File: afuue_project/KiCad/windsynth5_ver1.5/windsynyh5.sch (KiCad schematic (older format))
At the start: 35 parts, among them P1 SENSOR, P2 SPEAKER, P3 HEADPHONE, P4 EXT-POWER, P5 EXT, P6 AE-PAM8012, P7 I2C, P8 MIDI-TRS, U1 ESP32-DEVKIT-C, U2 TDA1543, U3 TDA1543

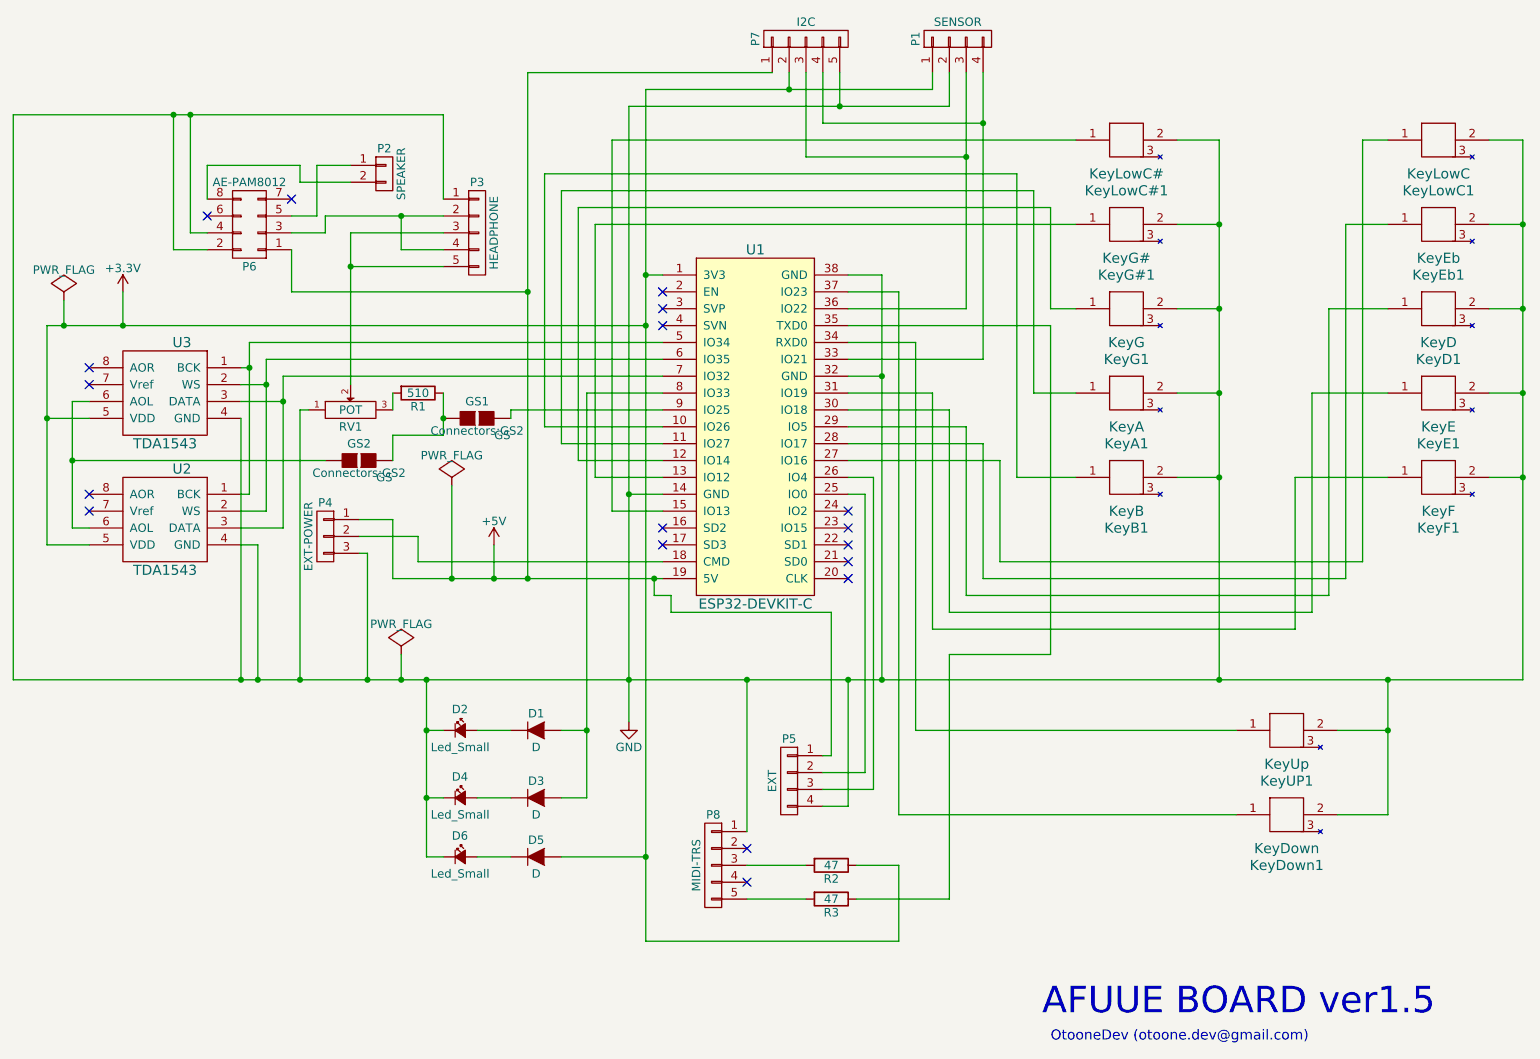
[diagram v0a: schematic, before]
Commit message: 現状のものを一旦コミット（KORG NTS-1対応含む）
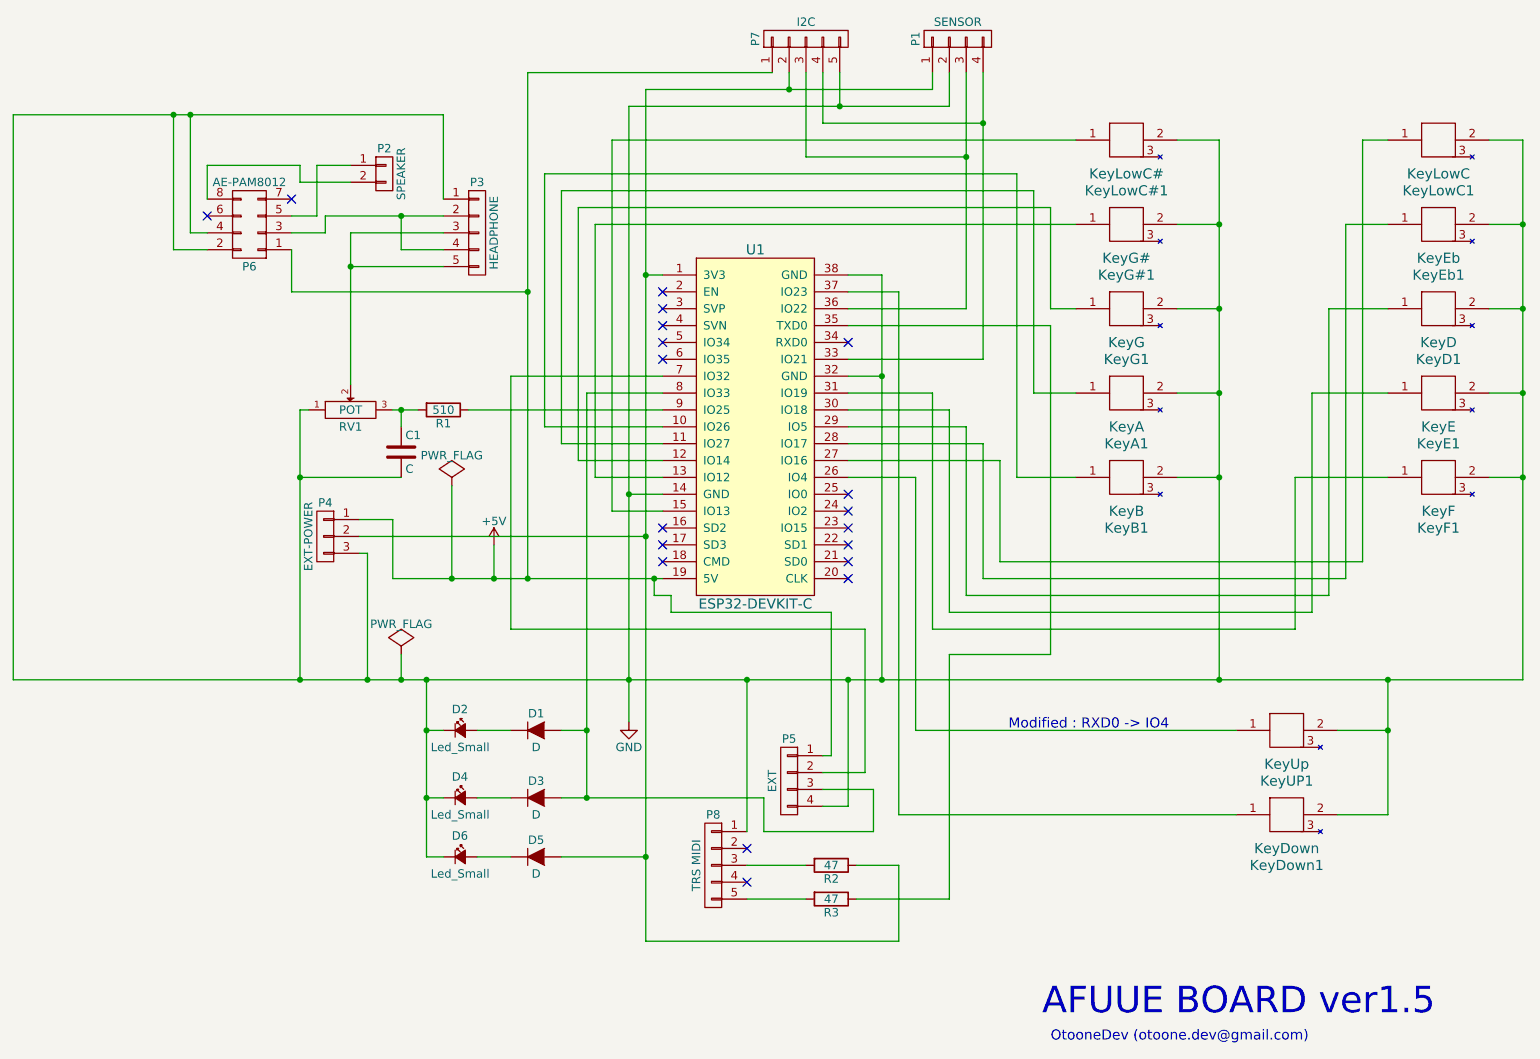
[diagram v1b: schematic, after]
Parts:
- removed GS1, GS2: GS, Connectors:GS2, symbol GS2
- removed U2: TDA1543, Housings_SOIC:SO-8_5.3x6.2mm_Pitch1.27mm, symbol TDA1543
- removed U3: TDA1543, Housings_DIP:DIP-8_W7.62mm, symbol TDA1543
- added C1: C, Pin_Headers:Pin_Header_Straight_1x02_Pitch2.54mm, symbol C
- P5: footprint Pin_Headers:Pin_Header_Straight_1x04_Pitch2.54mm -> Socket_Strips:Socket_Strip_Angled_1x04_Pitch2.54mm
- P8: value MIDI-TRS -> TRS MIDI
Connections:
- net +3V3 is gone; now on an unnamed net: D5.2 (A), P1.1 (P1), P7.2 (P2), R2.1, U1.1 (3V3)
- net GND: now also C1.2
- net at P4.2 (P2): no longer U1.18 (CMD)
- net at U1.25 (IO0): no longer P5.2 (P2)
- net at U1.26 (IO4): now also KeyUP1.1; no longer P5.3 (P3)
- net at U1.34 (RXD0): no longer KeyUP1.1
- net at U1.7 (IO32): now also P5.2 (P2)
- net at D1.2 (A), D3.2 (A), U1.8 (IO33): now also P5.3 (P3)
- net at U1.9 (IO25): now also R1.1
- net at R1.2, RV1.3: now also C1.1
- no-connect marks 18 -> 19
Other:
- note added: "Modified : RXD0 -> IO4"
- moved on the sheet: R1
